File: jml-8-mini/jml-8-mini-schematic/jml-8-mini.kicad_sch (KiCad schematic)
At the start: 19 parts, among them J1 Barrel_Jack, J2 Conn_01x09_Pin, J3 Conn_01x04_Pin, SW1 SW_DPDT_x2, U1 Z80CPU, U2 28HC64, U3 60L256, U4 Z80 CTC, U5 Z80 SIO

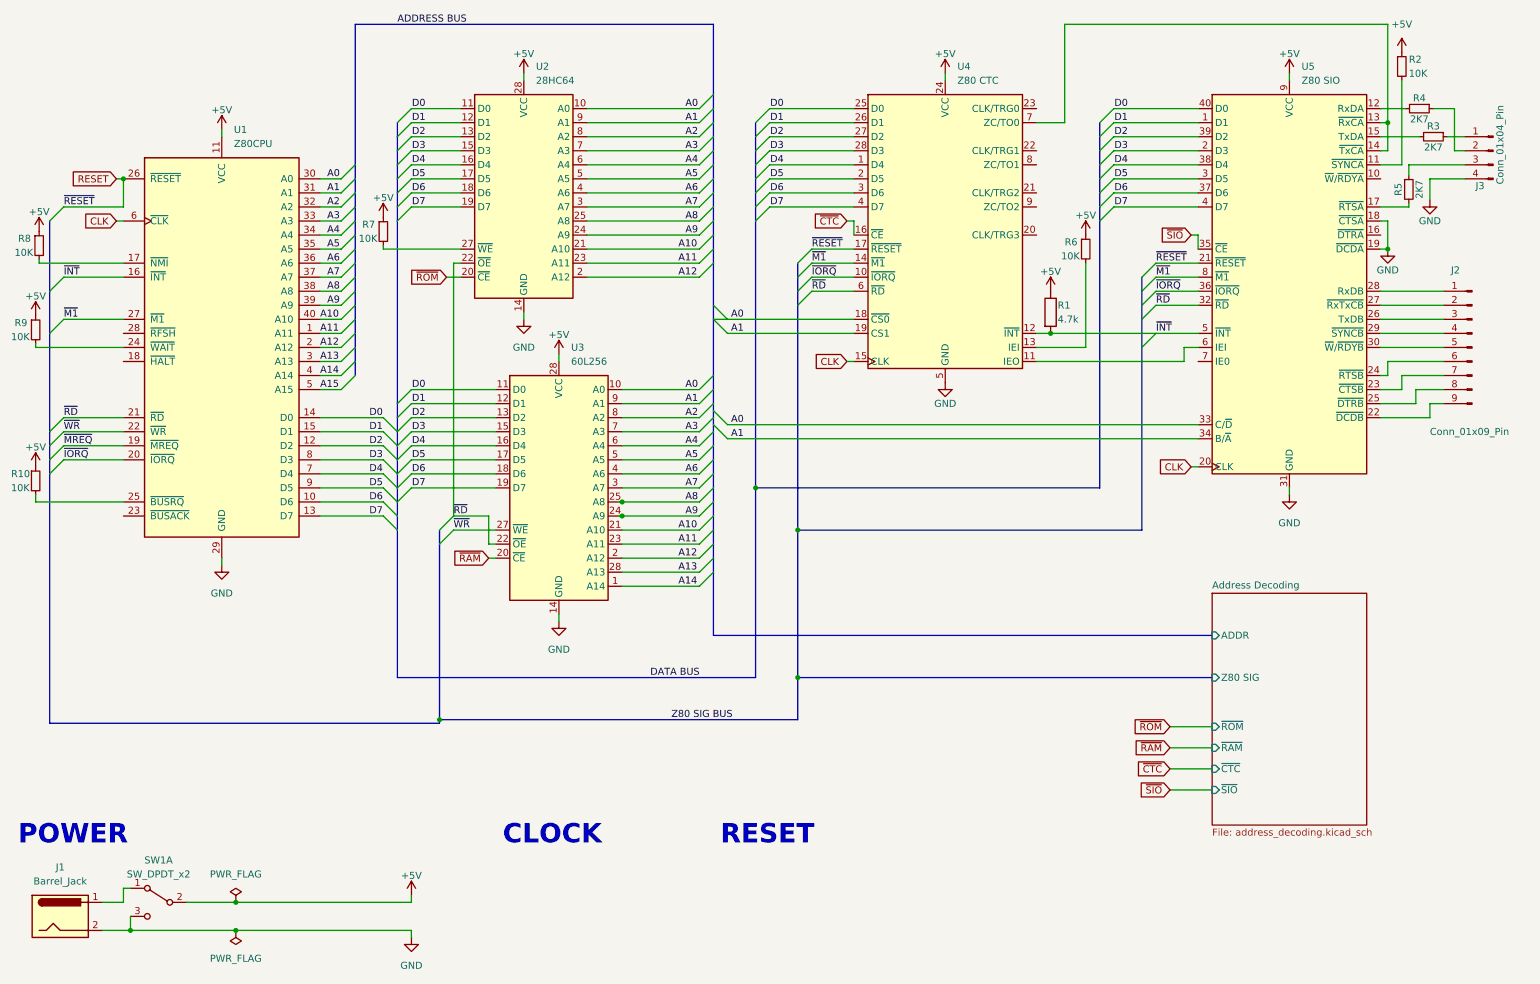
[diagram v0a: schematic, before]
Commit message: many changes to schematic to make more organized
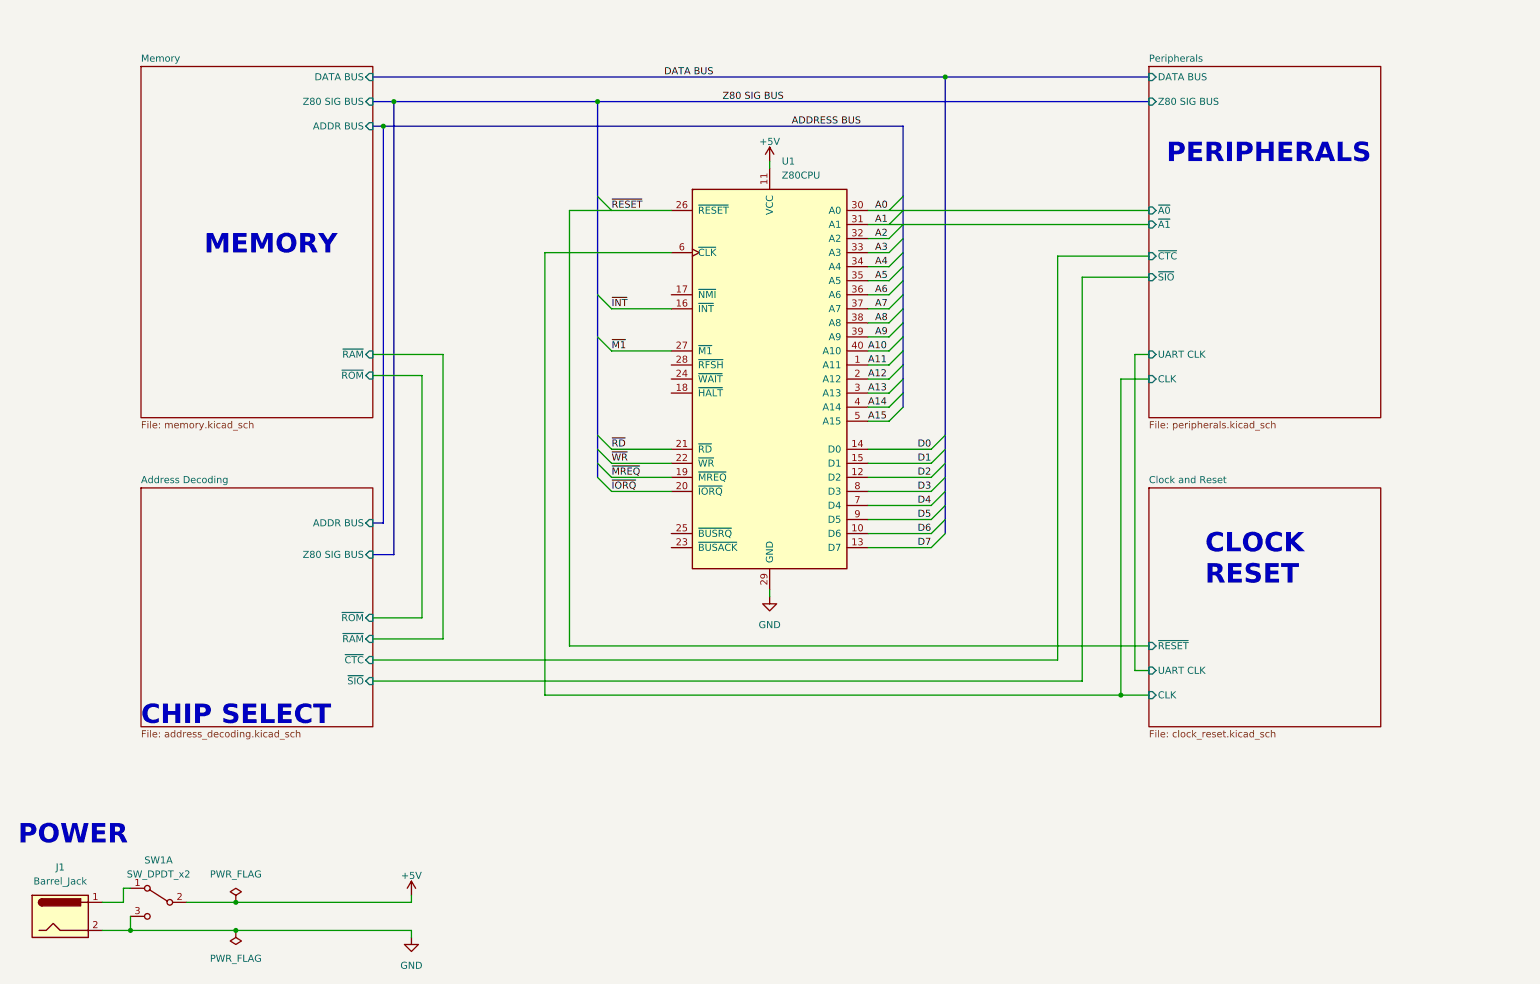
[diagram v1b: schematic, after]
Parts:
- removed J2: Conn_01x09_Pin, symbol Connector:Conn_01x09_Pin
- removed J3: Conn_01x04_Pin, symbol Connector:Conn_01x04_Pin
- removed R1: 4.7k, symbol Device:R
- removed R10, R2, R6, R7, R8, R9: 10K, symbol Device:R_Small
- removed R3, R4, R5: 2K7, symbol Device:R_Small
- removed U2: 28HC64, Package_DIP:DIP-28_W15.24mm_LongPads, symbol jml-8-mini-library:AT28HC64B
- removed U3: 60L256, Package_DIP:DIP-28_W15.24mm_LongPads, symbol jml-8-mini-library:MCM60L256AP85
- removed U4: Z80 CTC, symbol jml-8-mini-library:Z80_CTC
- removed U5: Z80 SIO, symbol jml-8-mini-library:Z80_SIO/0
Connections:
- net CLK renamed Clock and Reset/CLK
- net RESET renamed ~{RESET}
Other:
- added sheet Clock and Reset (clock_reset.kicad_sch)
- added sheet Memory (memory.kicad_sch)
- added sheet Peripherals (peripherals.kicad_sch)
- sheet Address Decoding ports: added ADDR BUS, Z80 SIG BUS; removed ADDR, Z80 SIG
- note added: "CHIP SELECT"
- note added: "CLOCK RESET"
- note added: "MEMORY"
- note added: "PERIPHERALS"
- note removed: "CLOCK"
- note removed: "RESET"
- moved on the sheet: U1
